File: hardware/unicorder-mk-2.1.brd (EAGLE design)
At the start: 38.2 x 32.3 mm, 13 parts, among them IC1 TINY85

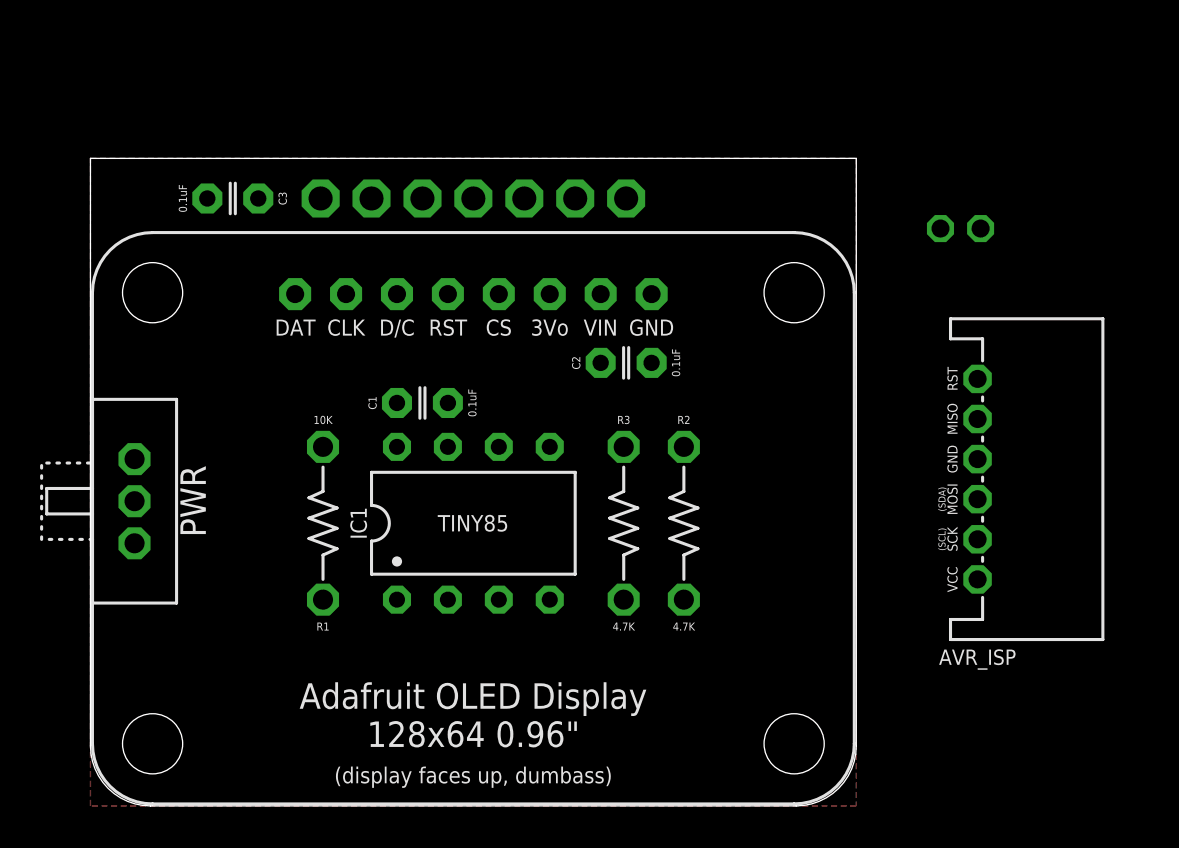
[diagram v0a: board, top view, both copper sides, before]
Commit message: alsdkfjkalsdf
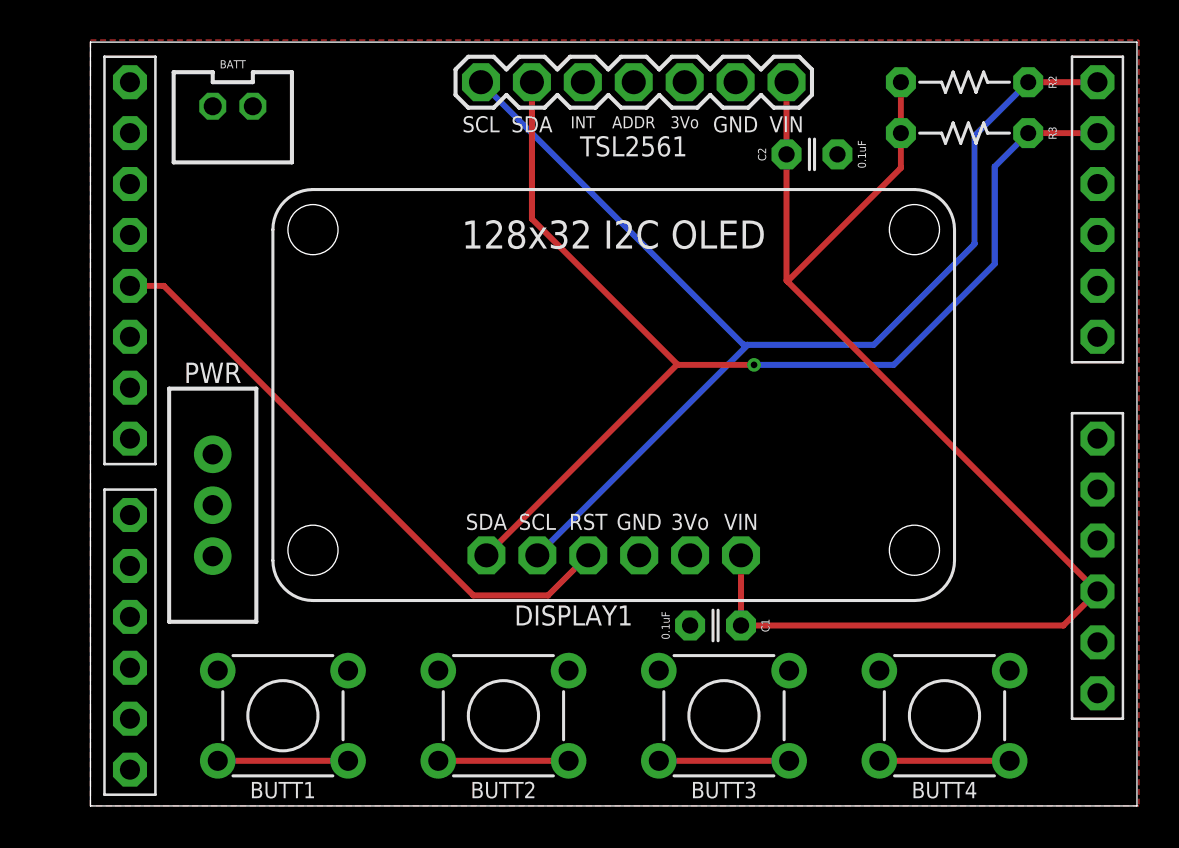
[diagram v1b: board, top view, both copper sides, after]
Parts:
- removed AVR_ISP: AVR_SPI_PRG_6AVR-JST-PTH-RA-I2C, A_butts:AVR-JST-6-PTH-RA-I2C
- removed C3: 0.1uF, A_butts:C025-024X044
- removed IC1: TINY85, A_butts:DIP08
- removed R1: 10K, A_butts:RESISTOR-AXIAL-PTH-7.62MM
- added BUTT1, BUTT2, BUTT3, BUTT4: SPST-NO-TACT6MM-PTH-SMALL-PADS, A_butts:DTS-6-SMALL-PADS
- added SHIELD: (no value), A_butts:ARDUINO_SHIELD_NOOUTLINE_INSIDE_SMALLER
- DISPLAY1: value ADAFRUIT_128X64_OLED -> ADAFRUIT_128X32_OLED_I2C; device A_butts:ADAFRUIT_128X64_OLED -> A_butts:ADAFRUIT_128X32_OLED_I2C_CLOSER
- PWR: value SWITCH-SPDTPTH-RA-2MM -> SWITCH-SPDTPTH-VERT-2.54MM; device A_butts:SPDT-RA-2MM -> A_butts:SWITCH-SPDT
- R2, R3: device A_butts:RESISTOR-AXIAL-PTH-7.62MM -> A_butts:RESISTOR-AXIAL-PTH-6.35MM
- moved BATT 36.8 mm to (7.00, 34.9), flipped to the top
- moved R2 26.1 mm to (43.5, 36.1), turned to 180 degrees
- moved R3 25.8 mm to (43.5, 33.6), turned to 180 degrees
- moved C1 18.4 mm to (31.1, 9.00), turned to 180 degrees
- moved DISPLAY1 14.8 mm to (26.0, 12.5)
- moved C2 13.9 mm to (35.9, 32.5)
- moved TSL2561 9.28 mm to (19.4, 36.1), flipped to the top
- moved PWR 3.91 mm to (6.00, 15.0), turned to 0 degrees
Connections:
- removed net MISO: AVR_ISP.MISO, IC1.6
- removed net MOSI/SDA: AVR_ISP.MOSI/SDA, DISPLAY1.DATA, IC1.5, R3.P$1, TSL2561.2
- removed net RST: AVR_ISP.RESET, IC1.1, R1.P$1
- removed net SCK/SCL: AVR_ISP.SCK, DISPLAY1.CLK, IC1.7, R2.P$1, TSL2561.1
- new net BUTT1: BUTT1.1, BUTT1.2
- new net BUTT2: BUTT2.1, BUTT2.2
- new net BUTT3: BUTT3.1, BUTT3.2
- new net BUTT4: BUTT4.1, BUTT4.2
- new net SCL: DISPLAY1.SCL, R2.P$1, SHIELD.A5, TSL2561.1
- new net SDA: DISPLAY1.SDA, R3.P$1, SHIELD.A4, TSL2561.2
- net DISPLAY_RST: now also SHIELD.D4; no longer IC1.2
- net GND: now also BUTT1.3, BUTT1.4, BUTT2.3, BUTT2.4, BUTT3.3, BUTT3.4, BUTT4.3, BUTT4.4, SHIELD.GND@0, SHIELD.GND@1; no longer AVR_ISP.GND, C3.2, IC1.4
- net VCC: now also SHIELD.5V; no longer AVR_ISP.VCC, C3.1, IC1.8, R1.P$2
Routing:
- net VCC: track 0.00 -> 66.1 mm
- net SCL: track 0.00 -> 59.6 mm
- net SDA: track 0.00 -> 59.2 mm, vias 0 -> 1
- net DISPLAY_RST: track 0.00 -> 30.1 mm
- net BUTT4: track 0.00 -> 6.50 mm
- net BUTT3: track 0.00 -> 6.50 mm
- net BUTT2: track 0.00 -> 6.50 mm
- net BUTT1: track 0.00 -> 6.50 mm
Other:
- board size 38.2 x 32.3 mm -> 52.2 x 38.1 mm
